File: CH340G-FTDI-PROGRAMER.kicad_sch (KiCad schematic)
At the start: 12 parts, among them J1 PINS, X1 12MHz

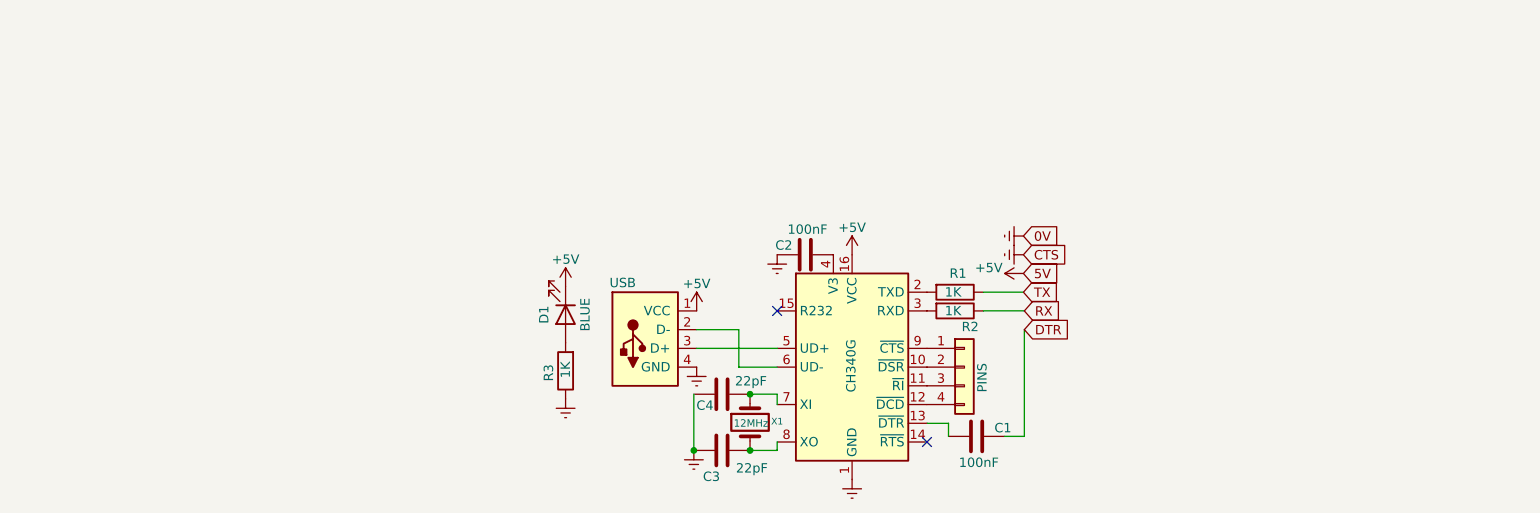
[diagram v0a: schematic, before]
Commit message: qq
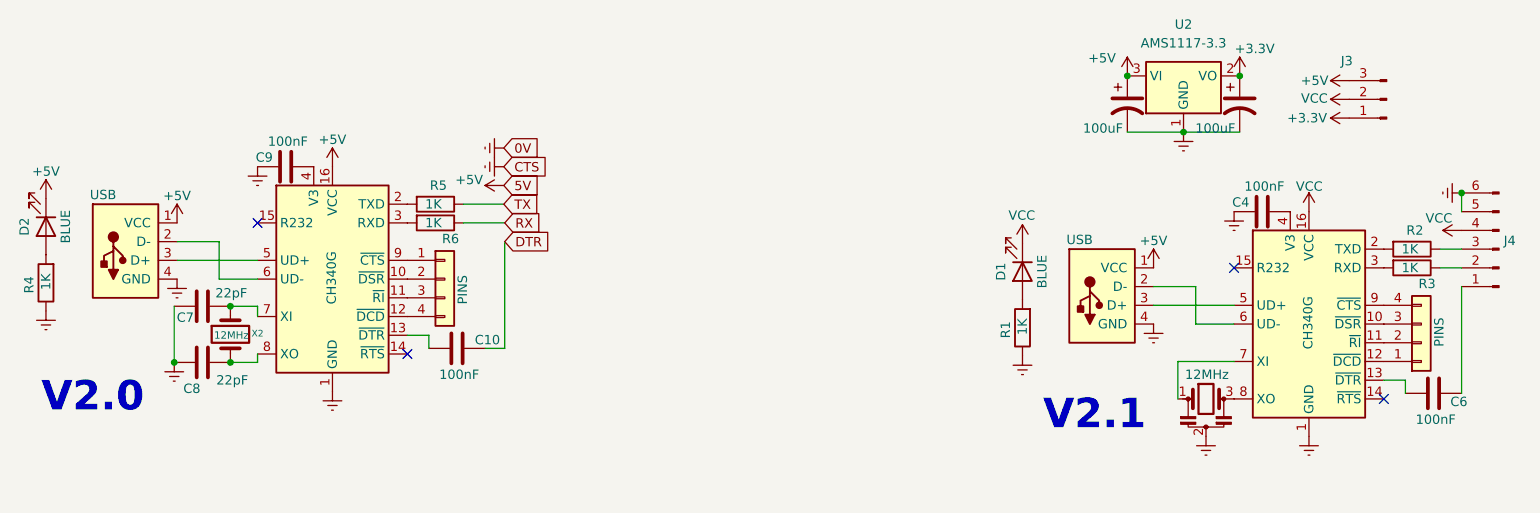
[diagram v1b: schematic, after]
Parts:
- removed C1, C2: 100nF, symbol Device:C
- removed C3: 22pF, symbol Device:C
- removed J1: PINS, symbol Connector_Generic_MountingPin:Conn_01x04_MountingPin
- removed J?: USB, symbol Connector:USB_A
- removed U?: CH340G, Package_SO:SOIC-16_3.9x9.9mm_P1.27mm, symbol Interface_USB:CH340G
- removed X1: 12MHz, symbol Device:Crystal
- added C1, C2: 100uF, Capacitor_SMD:C_1210_3225Metric_Pad1.33x2.70mm_HandSolder, symbol Device:C_Polarized_US
- added C10, C6, C9: 100nF, symbol Device:C
- added C7, C8: 22pF, symbol Device:C
- added D2: BLUE, symbol Device:LED
- added J1, J2: USB, symbol Connector:USB_A
- added J2, J3: PINS, symbol Connector_Generic_MountingPin:Conn_01x04_MountingPin
- added J3: Conn_01x03_Pin, symbol Connector:Conn_01x03_Pin
- added J4: Conn_01x06_Pin, symbol Connector:Conn_01x06_Pin
- added R4, R5, R6: 1K, symbol Device:R
- added U2 (x2): CH340G, Package_SO:SOIC-16_3.9x9.9mm_P1.27mm, symbol Interface_USB:CH340G
- added U2: AMS1117-3.3, Package_TO_SOT_SMD:SOT-223-3_TabPin2, symbol Regulator_Linear:AMS1117-3.3
- added X2: 12MHz, symbol Device:Crystal
- added Y1: 12MHz, Crystal:Resonator_SMD_Murata_CSTxExxV-3Pin_3.0x1.1mm, symbol Device:Resonator
- C4: value 22pF -> 100nF
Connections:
- net +5V: now also C1.1, D2.1 (K), J1.1 (VCC), J2.1 (VCC), J3.3 (Pin_3), U2.16 (VCC), U2.3 (VI); no longer D1.1 (K)
- net DTR: now also C10.1
- net Earth: now also C4.2, R1.1, C1.2, C2.2, C7.1, C8.1, C9.2, J1.4 (GND), J2.4 (GND), J4.5 (Pin_5), J4.6 (Pin_6), R4.1, U2.1 (GND), U2.1 (GND), U2.1 (GND), Y1.2; no longer C4.1, R3.1
- net RX: now also R6.1; no longer R2.1
- net TX: now also R5.1; no longer R1.1
- net at R1.2: now also D1.2 (A)
- net at R2.2: now also U2.2 (TXD)
- net at R3.2: now also U2.3 (RXD); no longer D1.2 (A)
- new net: J3.2 (Pin_2), U2.10 (~{DSR})
- new net: J3.3 (Pin_3), U2.11 (~{RI})
- new net: J3.4 (Pin_4), U2.12 (~{DCD})
- new net: C10.2, U2.13 (~{DTR})
- new net: R5.2, U2.2 (TXD)
- new net: R6.2, U2.3 (RXD)
- new net: C9.1, U2.4 (V3)
- new net: J2.3 (D+), U2.5 (UD+)
- new net: J2.2 (D-), U2.6 (UD-)
- new net: C7.2, U2.7 (XI), X2.1
- new net: C8.2, U2.8 (XO), X2.2
- new net: J3.1 (Pin_1), U2.9 (~{CTS})
- new net: D2.2 (A), R4.2
- new net: C6.1, J4.1 (Pin_1)
- new net: C6.2, U2.13 (~{DTR})
- new net: J1.2 (D-), U2.6 (UD-)
- new net: J1.3 (D+), U2.5 (UD+)
- new net: J2.1 (Pin_1), U2.12 (~{DCD})
- new net: J2.2 (Pin_2), U2.11 (~{RI})
- new net: J2.3 (Pin_3), U2.10 (~{DSR})
- new net: J2.4 (Pin_4), U2.9 (~{CTS})
- new net: J4.2 (Pin_2), R3.1
- new net: C4.1, U2.4 (V3)
- new net: U2.7 (XI), Y1.1
- new net: U2.8 (XO), Y1.3
- new net: J4.3 (Pin_3), R2.1
- new net +3.3V: C2.1, J3.1 (Pin_1), U2.2 (VO)
- new net VCC: D1.1 (K), J3.2 (Pin_2), J4.4 (Pin_4), U2.16 (VCC)
- no-connect marks 2 -> 4
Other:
- note added: "V2.0"
- note added: "V2.1"
